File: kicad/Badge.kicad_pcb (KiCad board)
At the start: 2 copper layers, 25 parts, among them SW1 SW_SPST, U1 LMC555xM

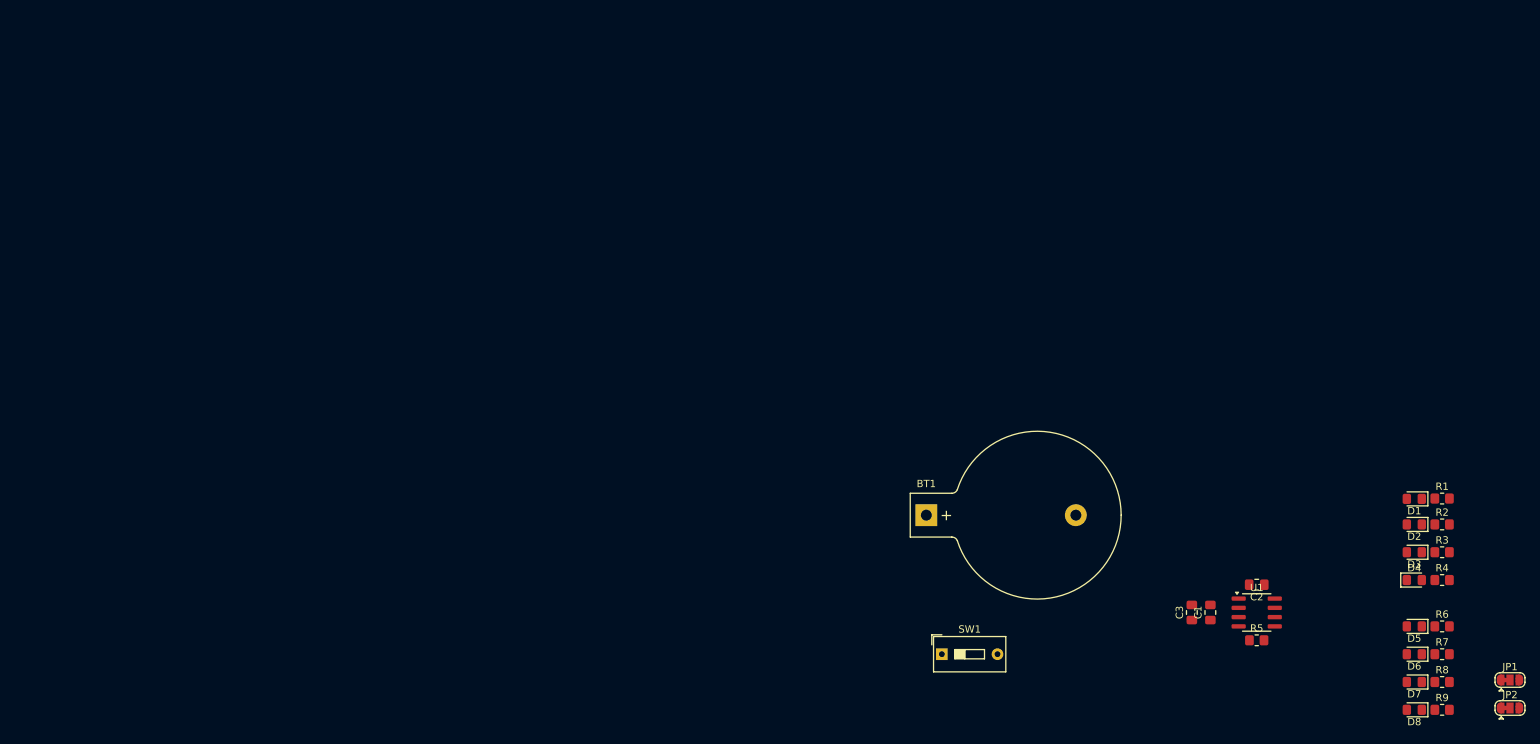
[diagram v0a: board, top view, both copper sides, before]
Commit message: routing 1
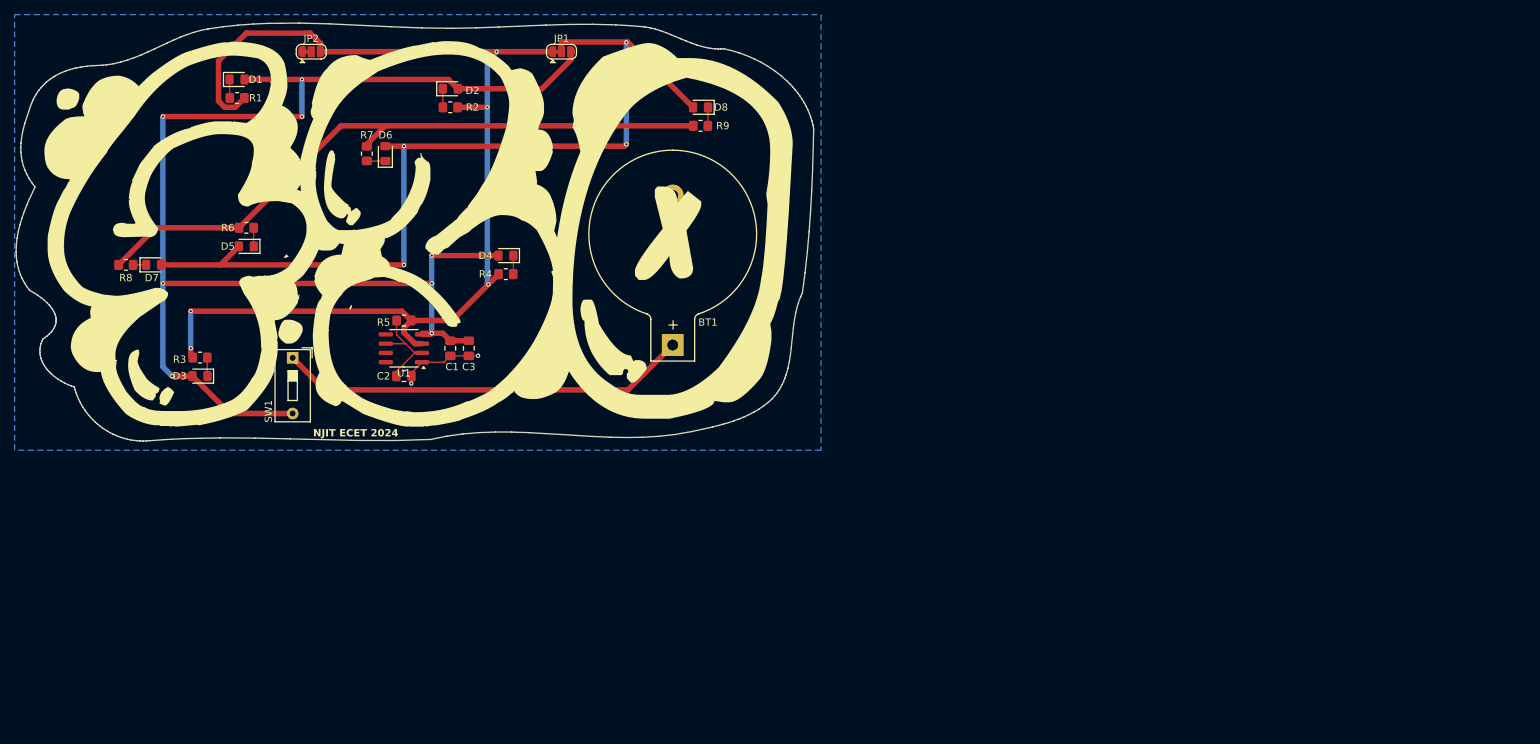
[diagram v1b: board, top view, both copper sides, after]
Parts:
- moved R8 189.2 mm to (52.1, 62.2), turned to 180 degrees
- moved JP2 187.2 mm to (77.5, 33.0)
- moved D7 181.9 mm to (55.9, 62.2), turned to 0 degrees
- moved R1 174.0 mm to (67.3, 39.4)
- moved R6 172.7 mm to (68.6, 57.1), turned to 180 degrees
- moved R3 172.3 mm to (62.2, 74.9), turned to 180 degrees
- moved D1 171.2 mm to (67.3, 36.8), turned to 0 degrees
- moved D5 168.3 mm to (68.6, 59.7)
- moved D3 168.1 mm to (62.2, 77.5)
- moved R7 162.5 mm to (85.1, 47.0), turned to 90 degrees
- moved D6 156.8 mm to (87.6, 47.0), turned to 90 degrees
- moved JP1 155.9 mm to (111.8, 33.0)
- moved R2 147.4 mm to (96.5, 40.6)
- moved D2 144.9 mm to (96.5, 38.1), turned to 0 degrees
- moved R4 134.9 mm to (104.1, 63.5), turned to 180 degrees
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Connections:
- net Net-(BT1-+) renamed /BAT
- net Net-(D5-A) renamed /PULSE2H
- net Net-(JP2-C) renamed /PULSE2L
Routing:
- net VCC: track 0.00 -> 191.7 mm, vias 0 -> 8
- net /PULSE: track 0.00 -> 152.4 mm, vias 0 -> 5
- net /PULSE2H: track 0.00 -> 123.2 mm, vias 0 -> 4
- net /PULSE2L: track 0.00 -> 90.5 mm
- net /BAT: track 0.00 -> 56.4 mm
- net /TR: track 0.00 -> 13.4 mm
- net GND: track 0.00 -> 11.6 mm, vias 0 -> 2
- net Net-(D1-K): track 0.00 -> 2.59 mm
- net Net-(D4-K): track 0.00 -> 2.59 mm
- net Net-(D8-K): track 0.00 -> 2.55 mm
- net Net-(D5-K): track 0.00 -> 2.55 mm
- net Net-(D3-K): track 0.00 -> 2.55 mm
- net Net-(D6-K): track 0.00 -> 2.55 mm
- net Net-(D2-K): track 0.00 -> 2.55 mm
- net Net-(D7-K): track 0.00 -> 1.78 mm
- added copper zone on B.Cu, net GND
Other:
- board outline added: 109.3 x 57.3 mm
- board text added: "NJIT ECET 2024"
